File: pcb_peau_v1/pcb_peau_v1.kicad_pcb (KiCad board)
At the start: 2 copper layers, 70 x 70 mm, 27 parts, among them J1 Conn_01x05, J2 Conn_01x05, J3 Conn_01x02, J4 Conn_02x08_Top_Bottom, J5 Conn_02x12_Top_Bottom, U2 TLC274, U3 CD74HC4067SM, U4 CD74HC4067SM, U5 CD74HC4067SM, U6 CD74HC4067SM, U7 TLC274, U8 TLC274, U9 TLC274

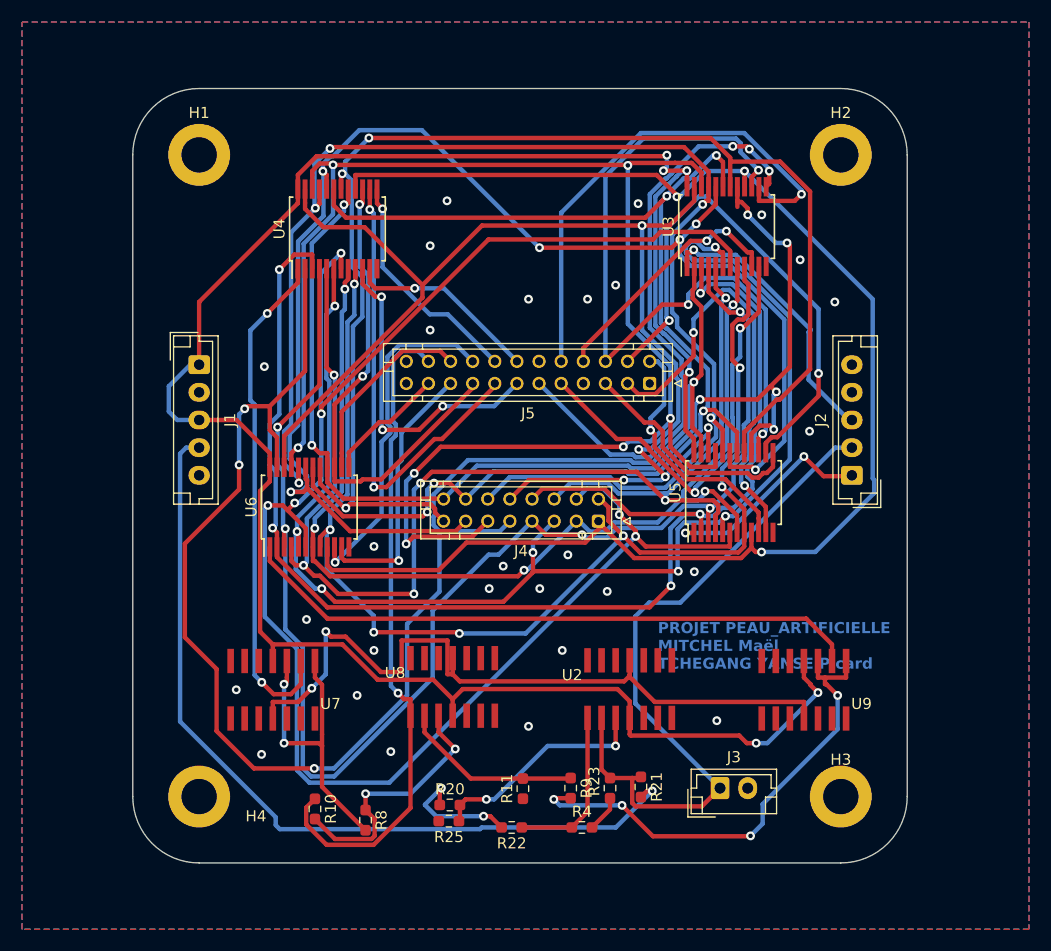
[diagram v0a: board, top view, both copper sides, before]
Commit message: PCB au bonnes normes (on y croit)
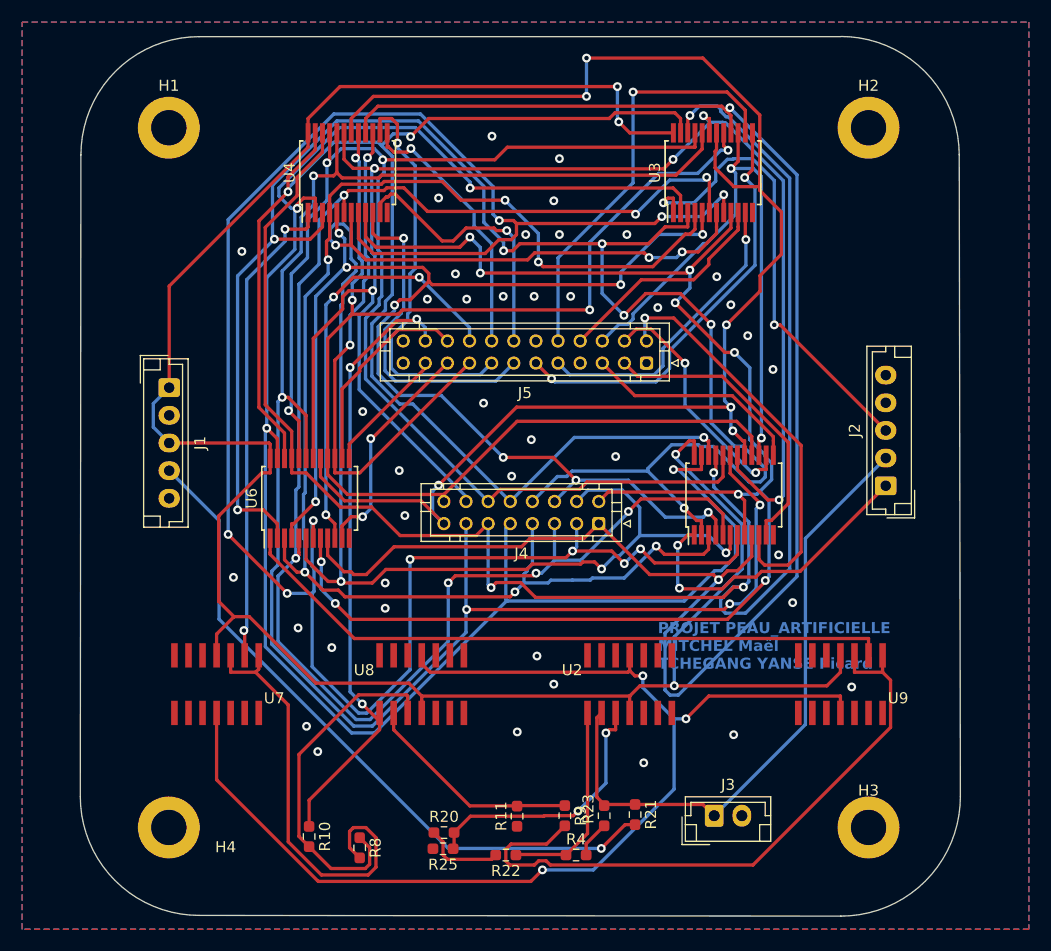
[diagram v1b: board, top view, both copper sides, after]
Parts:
- moved U4 5.16 mm to (191.4, 54.6)
- moved U7 5.11 mm to (179.6, 100.8)
- moved U3 5.02 mm to (224.4, 54.6)
- moved H4 3.91 mm to (175.3, 113.8)
- moved H3 3.75 mm to (238.5, 113.8)
- moved H1 3.68 mm to (175.3, 50.5)
- moved H2 3.51 mm to (238.5, 50.5)
- moved J1 3.41 mm to (175.3, 74.0)
- moved U9 3.34 mm to (236.0, 100.8)
- moved J2 3.20 mm to (240.1, 82.9)
- moved U8 2.81 mm to (198.1, 100.8)
- moved R11 2.55 mm to (206.7, 112.8)
- moved R4 2.55 mm to (212.1, 116.3)
- moved J3 2.55 mm to (224.6, 112.7)
- moved R10 2.55 mm to (187.9, 114.6)
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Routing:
- net Net-(J4-Pin_3): track 96.3 -> 187.5 mm, vias 5 -> 10
- net -5V: track 67.7 -> 106.2 mm, vias 2 -> 3
- net Net-(J4-Pin_13): track 130.3 -> 166.5 mm, vias 6 -> 5
- net Net-(J4-Pin_2): track 108.3 -> 141.9 mm, vias 7 -> 9
- net Net-(J4-Pin_4): track 163.2 -> 132.4 mm
- net Net-(J4-Pin_8): track 128.3 -> 158.0 mm, vias 5 -> 7
- net C1: track 48.1 -> 22.3 mm
- net Net-(J4-Pin_1): track 132.5 -> 158.0 mm, vias 3 -> 2
- net Net-(J4-Pin_5): track 121.5 -> 145.3 mm
- net Net-(J4-Pin_14): track 114.9 -> 138.0 mm
- net Net-(J4-Pin_10): track 116.2 -> 134.1 mm, vias 5 -> 3
- net Net-(J4-Pin_11): track 141.3 -> 158.3 mm, vias 7 -> 4
- net 2-ENTREE: track 25.6 -> 42.5 mm, vias 1 -> 2
- net Net-(J4-Pin_16): track 105.8 -> 122.7 mm, vias 7 -> 4
- net Net-(J4-Pin_9): track 150.2 -> 167.0 mm
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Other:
- board size 70 x 70 mm -> 79.5 x 79.5 mm
